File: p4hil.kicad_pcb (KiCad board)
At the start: 4 copper layers, 81.3 x 61 mm, 228 parts, among them J1 Conn_02x02_Odd_Even, J10 Conn_01x20, J11 Conn_01x20, J12 Conn_01x20, J13 USB_A_Stacked, J14 Conn_01x04, J15 Conn_01x20, J16 Conn_01x04, J17 Barrel_Jack_Switch, J18 Conn_02x05_Odd_Even, J19 HR871150C, J2 Conn_01x08, J20 Conn_02x04_Odd_Even, J21 Conn_01x06, J3 USB_C_Receptacle_USB2.0_16P, J4 Conn_01x10, J5 Conn_01x20, J6 Conn_01x20, J7 Conn_01x20, J8 Conn_01x02, J9 Conn_01x06, SW1 SW_Push, SW2 SW_Push, U1 W25Q128JVS, U10 TLV62569DBV, U11 MT9700_SY6280, U3 TLV62569DBV, U4 IPGRI, U5 PI4IOE5V9535ZDEX, U6 INA219AxD, U7 CH334F, U8 MT9700_SY6280, U9 MT9700_SY6280, Y1 40MHz(+-10 ppm) C501798, Y2 25Mhz 12pf, Y3 12MHz

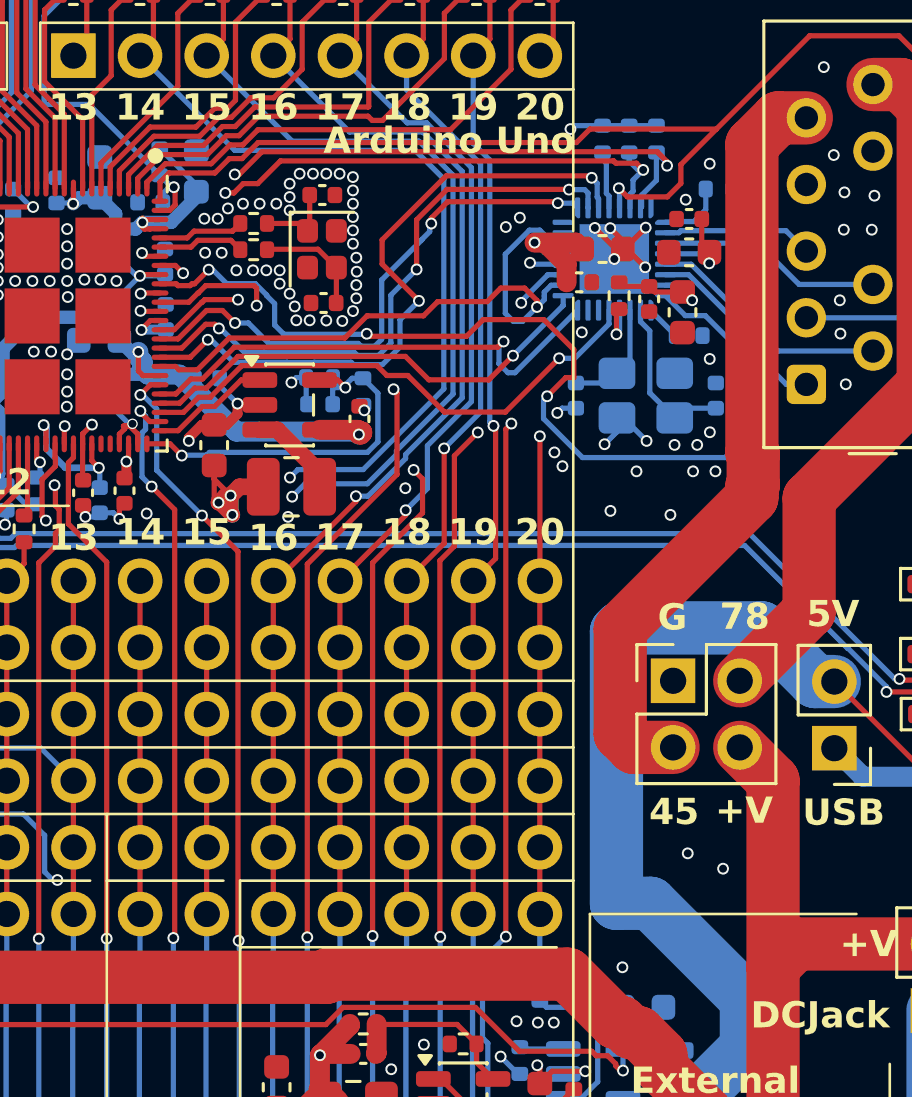
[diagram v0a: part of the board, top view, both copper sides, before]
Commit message: v1
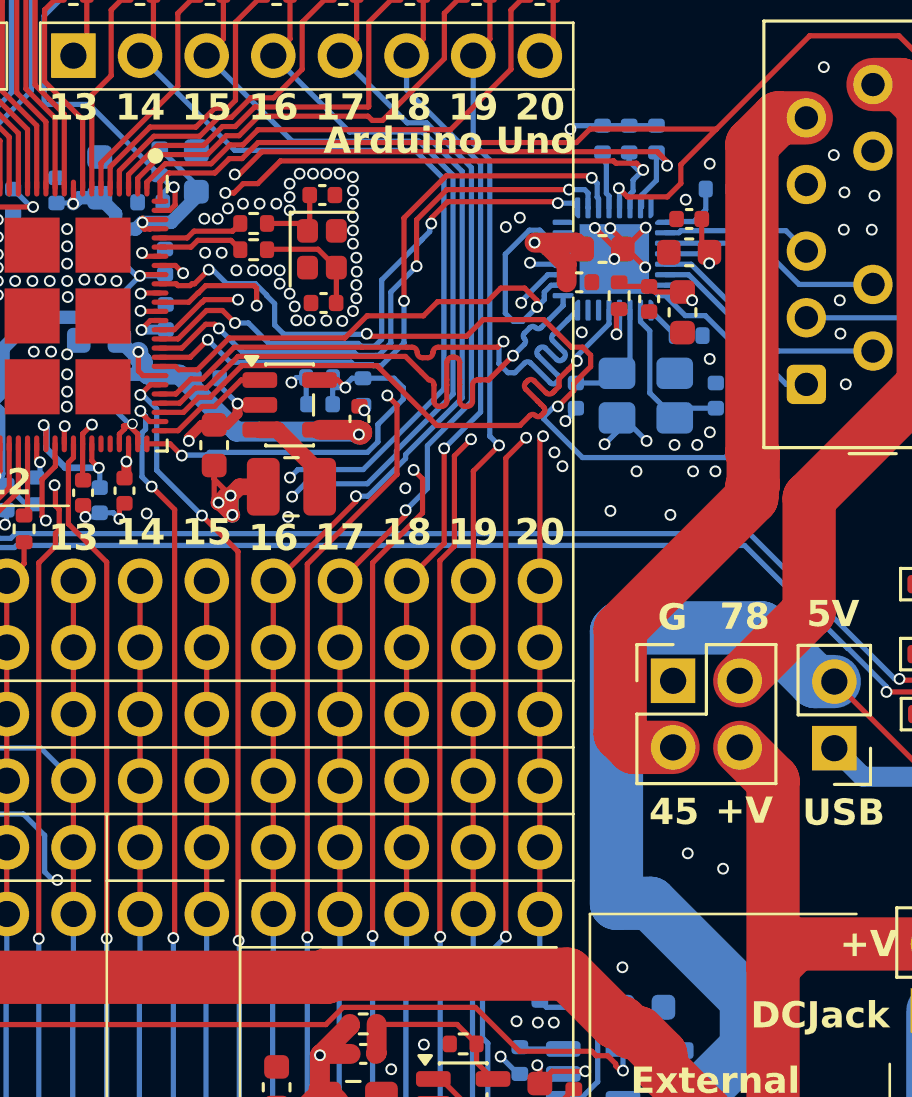
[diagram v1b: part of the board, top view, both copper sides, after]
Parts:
- R16, R17: value 220 -> 4.7K
- R18: value 470 -> 47K
- R26, R93: value 2.2K -> 4.7K
- R73: value 470 -> 4.7K
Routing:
- net /Ethernet/RMII_TXD0: track 18.0 -> 23.4 mm
- net /Ethernet/RMII_TXD1: track 19.0 -> 23.4 mm
- net /Ethernet/RMII_TXEN: track 20.5 -> 23.3 mm
- net /P4/FB_DCDC: track 15.7 -> 17.2 mm
- net /Ethernet/RMII_CRSDV: track 25.4 -> 24.2 mm
- net /DeviceUnderTest/T19i: track 40.3 -> 39.5 mm
- net /PHY_RESETN: track 37.6 -> 38.3 mm
